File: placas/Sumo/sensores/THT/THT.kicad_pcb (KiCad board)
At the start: 2 copper layers, 37.1 x 56.6 mm, 12 parts, among them J1 Conn_01x02_Male, J2 Control Sensores, U1 Mini360

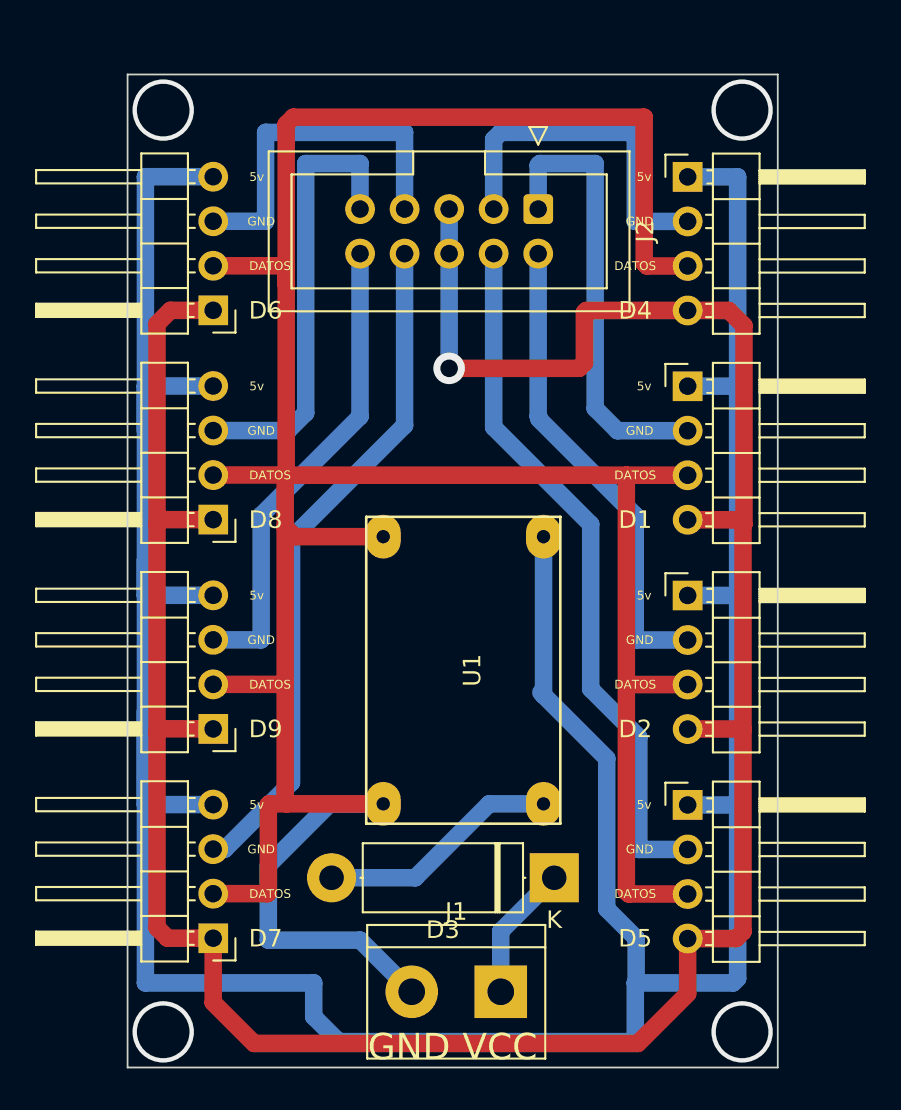
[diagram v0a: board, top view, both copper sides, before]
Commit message: MAI
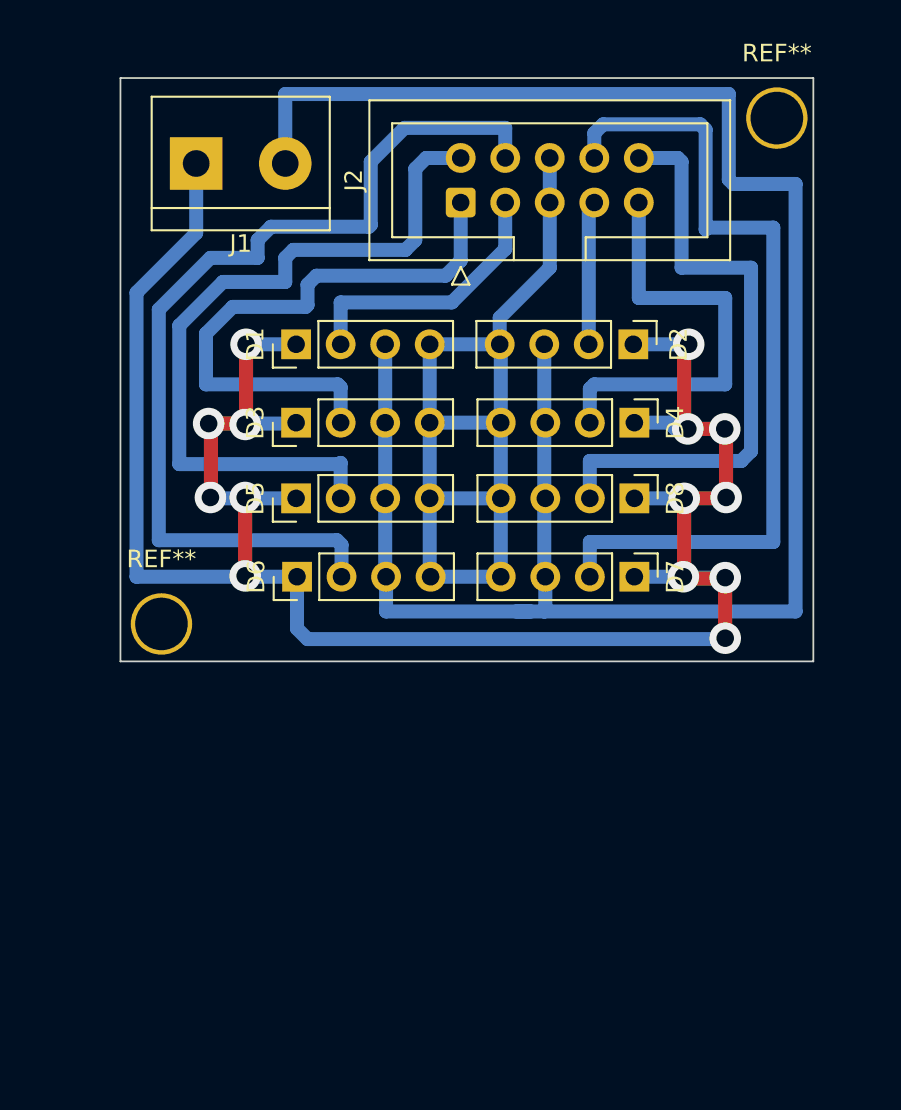
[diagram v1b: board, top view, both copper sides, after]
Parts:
- removed the D3 at (43.9, 60.6)
- removed D9: Conn_01x04_Male, Connector_PinHeader_2.54mm:PinHeader_1x04_P2.54mm_Horizontal
- removed U1: Mini360, Mini360_step-down:Mini360_step-down
- added D5: Conn_01x04_Male, Connector_PinHeader_2.54mm:PinHeader_1x04_P2.54mm_Vertical, F.Cu at (29.2, 38.9)
- added REF**: MountingHole_2.7mm_Pad, MountingHole:MountingHole_2.7mm_Pad, F.Cu at (21.5, 46.1)
- added REF**: MountingHole_2.7mm_Pad, MountingHole:MountingHole_2.7mm_Pad, F.Cu at (56.6, 17.2)
- D1, D2, D6, D7, D8: footprint Connector_PinHeader_2.54mm:PinHeader_1x04_P2.54mm_Horizontal -> Connector_PinHeader_2.54mm:PinHeader_1x04_P2.54mm_Vertical
- D3: renamed from D4; footprint Connector_PinHeader_2.54mm:PinHeader_1x04_P2.54mm_Horizontal -> Connector_PinHeader_2.54mm:PinHeader_1x04_P2.54mm_Vertical
- D4: renamed from D5; footprint Connector_PinHeader_2.54mm:PinHeader_1x04_P2.54mm_Horizontal -> Connector_PinHeader_2.54mm:PinHeader_1x04_P2.54mm_Vertical
- moved J1 50.3 mm to (23.5, 19.8), turned to 0 degrees
- moved D7 31.7 mm to (48.5, 43.4), turned to -90 degrees
- moved D3 26.4 mm to (29.2, 34.6), turned to 90 degrees
- moved D8 24.1 mm to (48.5, 38.9), turned to -90 degrees
- moved D1 22.5 mm to (29.2, 30.1), turned to 90 degrees
- moved D4 22.0 mm to (48.5, 34.6), turned to -90 degrees
- moved D6 15.9 mm to (29.2, 43.4), turned to 90 degrees
- moved D2 14.7 mm to (48.4, 30.1), turned to -90 degrees
- moved J2 4.44 mm to (38.6, 22.0), turned to 90 degrees
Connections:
- D6 pad 1: /38Kh -> /5v
- D6 pad 2: /gnd -> /data6
- D6 pad 3: /data5 -> /gnd
- D6 pad 4: /5v -> /38Kh
- D7 pad 1: /38Kh -> /5v
- D7 pad 2: /gnd -> /data7
- D7 pad 3: /data8 -> /gnd
- D7 pad 4: /5v -> /38Kh
- D8 pad 1: /38Kh -> /5v
- D8 pad 2: /gnd -> /data8
- D8 pad 3: /data6 -> /gnd
- D8 pad 4: /5v -> /38Kh
- J1 pad 1: Net-(D3-Pad1) -> /5v
- J2 pad 1: /data2 -> /data1
- J2 pad 10: /data7 -> /data8
- J2 pad 2: /data3 -> /data5
- J2 pad 3: /data1 -> /data2
- J2 pad 4: /data4 -> /data6
- J2 pad 7: /data5 -> /data3
- J2 pad 8: /data8 -> /data7
- J2 pad 9: /data6 -> /data4
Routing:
- net /38Kh: track 157.7 -> 54.6 mm, vias 1 -> 0
- net /5v: track 196.3 -> 133.3 mm, vias 0 -> 14
- net /gnd: track 179.9 -> 117.2 mm
- net /data6: track 25.6 -> 54.0 mm
- net /data5: track 20.4 -> 42.4 mm
- net /data7: track 27.1 -> 48.1 mm
- net /data3: track 27.3 -> 8.22 mm
- net /data4: track 40.2 -> 25.1 mm
- net Net-(D3-Pad2): track 13.8 -> 0.00 mm
- net /data1: track 20.3 -> 32.9 mm
- net /data2: track 25.6 -> 15.7 mm
- net Net-(D3-Pad1): track 7.76 -> 0.00 mm
- net /data8: track 38.9 -> 34.6 mm
- net (no net): vias 4 -> 0
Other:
- board size 37.1 x 56.6 mm -> 39.5 x 33.3 mm
- board text removed: "5v"
- board text removed: "DATOS"
- board text removed: "GND"
- board text removed: "VCC"
